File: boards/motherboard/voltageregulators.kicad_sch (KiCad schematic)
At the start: 4 parts, among them U6 AMS1117-3.3

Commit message: feat: assign footprints
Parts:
- C48, C49: footprint (none) -> Capacitor_SMD:C_0603_1608Metric
- C50: footprint (none) -> Capacitor_SMD:CP_Elec_4x5.4
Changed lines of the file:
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@@
       (effects (font (size 1.27 1.27)) (justify left))
     )
-    (property "Footprint" "" (id 2) (at 61.9252 41.91 0)
+    (property "Footprint" "Capacitor_SMD:CP_Elec_4x5.4" (id 2) (at 61.9252 41.91 0)
       (effects (font (size 1.27 1.27)) hide)
     )
@@
       (effects (font (size 1.27 1.27)) (justify left))
     )
-    (property "Footprint" "" (id 2) (at 31.4452 41.91 0)
+    (property "Footprint" "Capacitor_SMD:C_0603_1608Metric" (id 2) (at 31.4452 41.91 0)
       (effects (font (size 1.27 1.27)) hide)
     )
@@
       (effects (font (size 1.27 1.27)) (justify left))
     )
-    (property "Footprint" "" (id 2) (at 51.7652 41.91 0)
+    (property "Footprint" "Capacitor_SMD:C_0603_1608Metric" (id 2) (at 51.7652 41.91 0)
       (effects (font (size 1.27 1.27)) hide)
     )

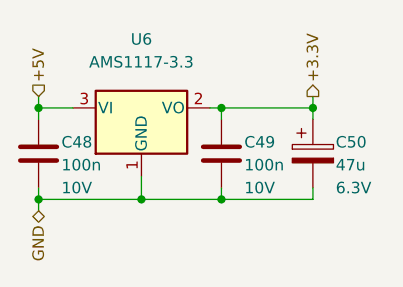
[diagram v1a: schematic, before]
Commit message: feat: first release of motherboard
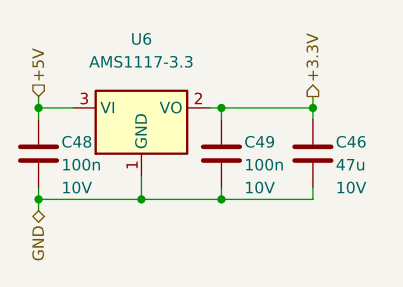
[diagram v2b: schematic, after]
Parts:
- removed C50: 47u, Capacitor_SMD:CP_Elec_4x5.4, symbol Device:C_Polarized
- added C46: 47u, Capacitor_SMD:C_0603_1608Metric, symbol Device:C
- C48, C49: LCSC PN (none) -> C14663
- U6: LCSC PN (none) -> C6186
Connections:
- net +3.3V: now also C46.1
- net GND: now also C46.2

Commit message: feat: revised motherboard
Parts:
- C46: footprint Capacitor_SMD:C_0603_1608Metric -> Capacitor_SMD:C_1206_3216Metric
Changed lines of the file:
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@@
 			)
 		)
-		(property "Footprint" "Capacitor_SMD:C_0603_1608Metric"
+		(property "Footprint" "Capacitor_SMD:C_1206_3216Metric"
 			(at 61.9252 41.91 0)
 			(effects
